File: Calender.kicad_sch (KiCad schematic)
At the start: 37 parts, among them J1 Conn_01x09, J2 USB_C_Receptacle_USB2.0_16P, J3 Power, SW1 RotaryEncoder_Switch, SW2 SW_Push, SW3 SW_Push, SW4 SW_Push, U1 ATSAMD21G18A-A, U3 MCP73871, U4 AMS1117-3.3, U5 ESP-WROOM-02

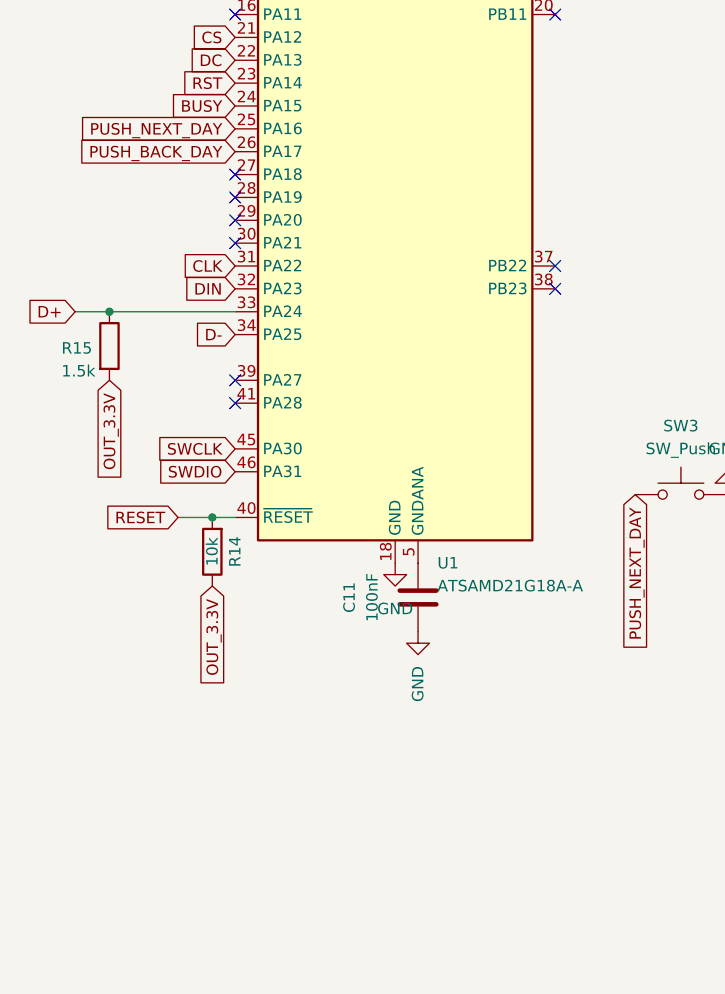
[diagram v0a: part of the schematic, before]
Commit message: Fixed PCB changes/errors
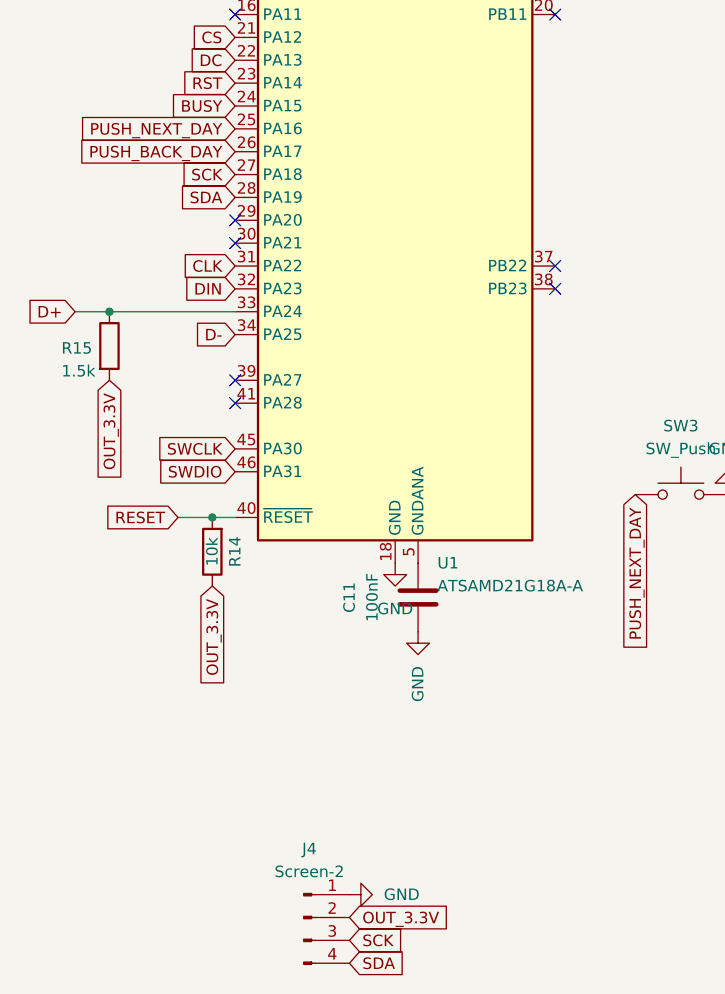
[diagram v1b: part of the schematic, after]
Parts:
- added J4: Screen-2, Connector_PinHeader_2.54mm:PinHeader_1x04_P2.54mm_Vertical, symbol Connector:Conn_01x04_Pin
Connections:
- net GND: now also J4.1 (Pin_1)
- net OUT_3.3V: now also J4.2 (Pin_2)
- net SCK: now reaches U1.27 (PA18)
- net SCK: now also J4.3 (Pin_3)
- net SDA: now reaches U1.28 (PA19)
- net SDA: now also J4.4 (Pin_4)
- no-connect marks 32 -> 30
